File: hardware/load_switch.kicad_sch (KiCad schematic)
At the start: 18 parts, among them Q1 IPT015N10N5, Q2 IPT015N10N5, Q3 IPT015N10N5, Q4 IPT015N10N5, Q5 IPT015N10N5, Q6 IPT015N10N5

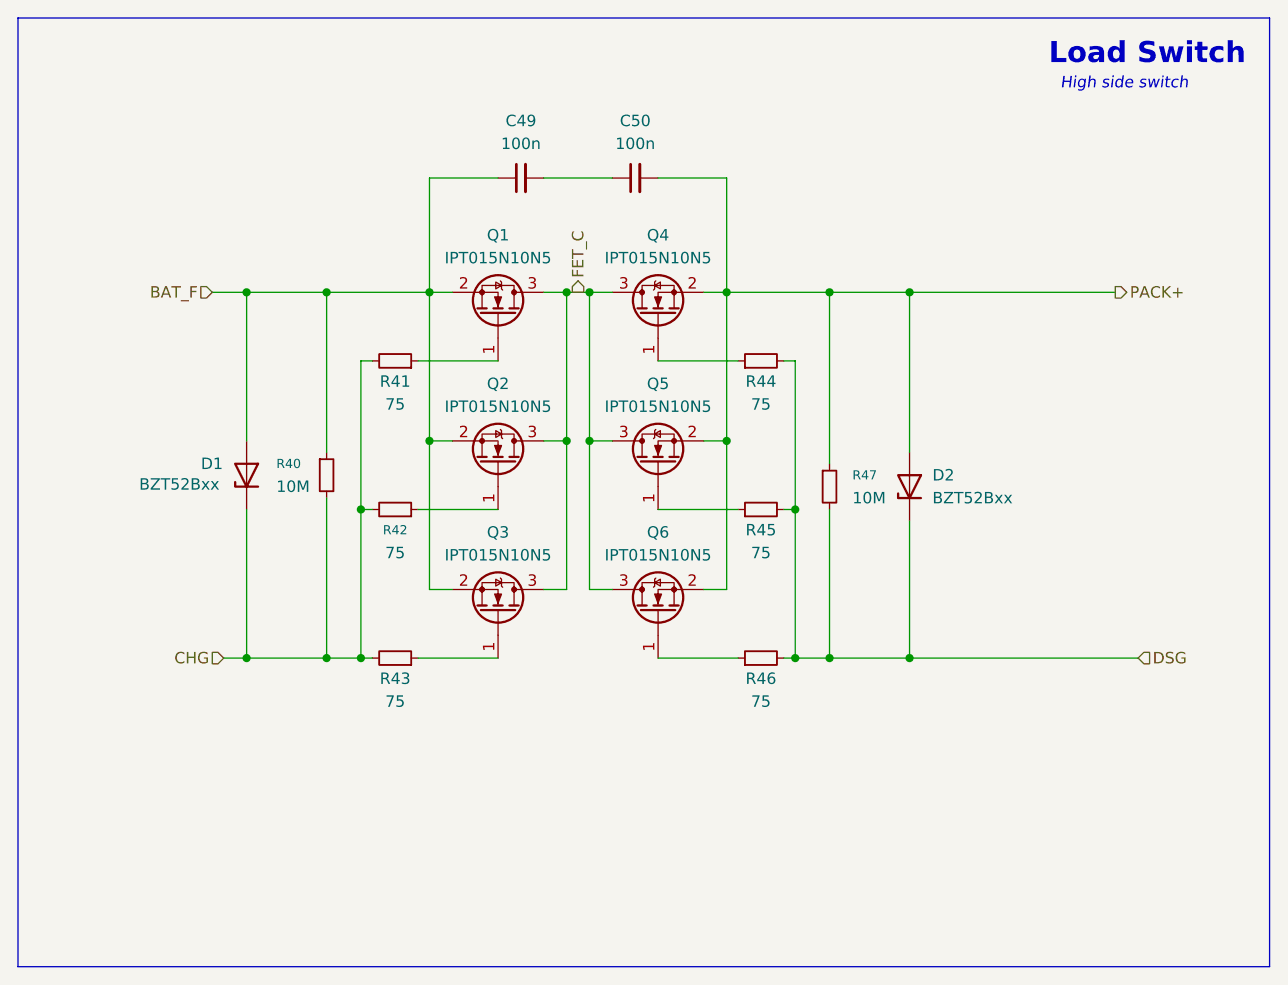
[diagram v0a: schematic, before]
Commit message: Changed to charge only BMS
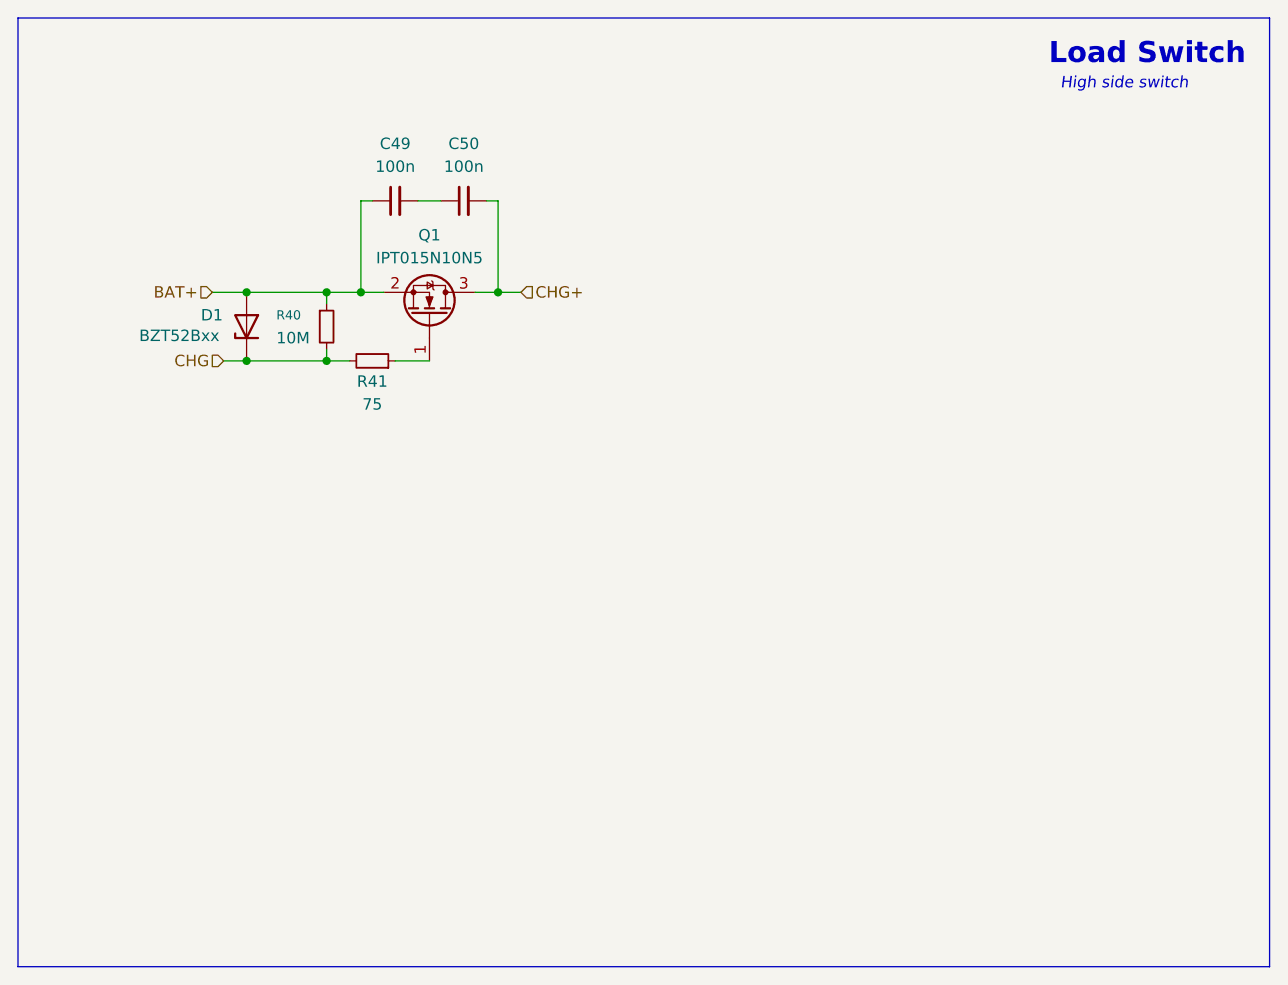
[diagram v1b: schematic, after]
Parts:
- removed D2: BZT52Bxx, Diode_SMD:D_SOD-123F, symbol Diode:BZT52Bxx
- removed Q2, Q3, Q4, Q5, Q6: IPT015N10N5, Package_TO_SOT_SMD:Infineon_PG-HSOF-8-1_ThermalVias, symbol Transistor_FET:IPT015N10N5
- removed R42, R43, R44, R45, R46: 75, Capacitor_SMD:C_0402_1005Metric, symbol Device:R_Small
- removed R47: 10M, Resistor_SMD:R_0402_1005Metric, symbol Device:R_Small
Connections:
- net PACK+ is gone; now on net CHG+: C50.2
- net BAT_F renamed BAT+
- net FET_C renamed CHG+
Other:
- moved on the sheet: C49, C50, D1, Q1, R40, R41
